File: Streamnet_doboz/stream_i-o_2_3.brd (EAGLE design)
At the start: 192 x 74.5 mm, 225 parts, among them IC1 SCT21SOP16, IC12 LD117AS33TR, IC3 BEM_VEDO, IC4 7805TV, J1 PIN1-2, Q1 20MHz, T1 BD242, T10 BD242, T11 BD242, T12 BD242, T13 BD242, T14 BD242, T15 BD242, T16 BD242, T17 BC858, T2 BD242, T3 BD242, T4 BD242, T5 BD242, T6 BD242, T7 BD242, T8 BD242, T9 BD242, U1 MAX232SOIC16, U2 PIC32MX250F128B-I_SS

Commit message: stream_haladás
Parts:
- removed U$2, U$3, U$4: SCT21SOP16, StarChips:SOP16
- added U$1, U$10, U$7, U$8, U$9: SCT2167SSOP, SCT2167:SSOP
- moved R16 288.9 mm to (-168.9, 33.8), flipped to the bottom
- moved D20 288.6 mm to (-168.8, 37.5), flipped to the bottom
- moved LED16 287.7 mm to (-168.3, 35.7), flipped to the bottom
- moved ZOLD_2P8 281.2 mm to (-165.0, 10.7), flipped to the bottom
- moved ZOLD_4P16 281.2 mm to (-165.0, 24.5), flipped to the bottom
- moved T16 273.7 mm to (-161.3, 27.3), flipped to the top
- moved D19 262.9 mm to (-155.9, 36.8), flipped to the bottom
- moved R46 259.1 mm to (-154.0, 2.22), flipped to the top
- moved R47 259.1 mm to (-154.0, 4.76), flipped to the top
- moved ZOLD_2P7 257.2 mm to (-153.0, 10.7), flipped to the bottom
- moved ZOLD_4P15 257.2 mm to (-153.0, 24.5), flipped to the bottom
- moved LED15 256.5 mm to (-152.7, 34.0), flipped to the bottom
- moved T15 253.4 mm to (-151.1, 38.7), flipped to the top
- moved D31 250.8 mm to (-149.9, 17.1), flipped to the top
- moved D32 250.8 mm to (-149.9, 14.8), flipped to the top
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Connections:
- removed net N$102: OK4.13, U$3.6
- removed net N$136: U$3.14, U$4.2
- new net 01_GND: U$10.1, U$7.1, U$8.1, U$9.1
- new net 16_VDD: U$10.16, U$7.16, U$8.16, U$9.16
- new net N$97: OK4.13, U$7.6
- net +3V3: now also U$1.16; no longer U$2.16, U$3.16, U$4.16
- net CHECK: no longer U$4.14
- net CLK: now also U$1.3; no longer U$2.3, U$3.3, U$4.3
- net GND: now also U$1.1, U$1.13; no longer U$2.1, U$2.13, U$3.1, U$3.13, U$4.1, U$4.13
- net LABE: now also U$1.4; no longer U$2.4, U$3.4, U$4.4
- net N$100: now also U$8.11; no longer U$4.11
- net N$101: now also U$7.5; no longer U$3.5
- net N$103: now also U$7.7; no longer U$3.7
- net N$104: now also U$7.8; no longer U$3.8
- net N$113: now also U$8.12; no longer U$4.12
- net N$127: now also U$8.5; no longer U$4.5
- net N$128: now also U$8.6; no longer U$4.6
- net N$129: now also U$8.7; no longer U$4.7
- net N$130: now also U$8.8; no longer U$4.8
- net N$131: no longer U$4.15
- net N$132: no longer U$3.15
- net N$133: now also U$1.15; no longer U$2.15
- net N$134: now also U$1.2; no longer U$2.2
- net N$135: now also U$1.14; no longer U$2.14, U$3.2
- net N$64: now also U$1.9; no longer U$2.9
- net N$65: now also U$1.10; no longer U$2.10
- net N$66: now also U$1.11; no longer U$2.11
- net N$67: now also U$1.12; no longer U$2.12
- net N$76: now also U$8.9; no longer U$4.9
- net N$77: now also U$1.5; no longer U$2.5
- net N$78: now also U$1.6; no longer U$2.6
- net N$79: now also U$1.7; no longer U$2.7
- net N$80: now also U$1.8; no longer U$2.8
- net N$88: now also U$7.9; no longer U$3.9
- net N$89: now also U$7.10; no longer U$3.10
- net N$90: now also U$7.11; no longer U$3.11
- net N$91: now also U$7.12; no longer U$3.12
- net N$96: now also U$8.10; no longer U$4.10
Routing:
- net LABE: track 302.0 -> 142.3 mm, vias 5 -> 2
- net N$135: track 124.6 -> 0.00 mm, vias 2 -> 0
- net N$136: track 115.8 -> 0.00 mm, vias 2 -> 0
- net GND: track 909.1 -> 899.7 mm
- net +3V3: track 376.9 -> 367.8 mm
- net N$102: track 5.63 -> 0.00 mm
- net N$97: track 0.00 -> 5.04 mm
- net CLK: track 280.3 -> 276.1 mm
- net N$130: track 7.50 -> 3.89 mm
- net N$103: track 6.90 -> 3.61 mm
- net N$79: track 6.90 -> 3.77 mm
- net N$133: track 11.6 -> 9.51 mm
- net N$132: track 3.95 -> 2.08 mm
- net N$131: track 4.80 -> 3.30 mm
- net N$89: track 40.4 -> 39.0 mm
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- added copper zone on layer 1, net GND
- removed copper zone on layer 16, net GND
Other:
- board size 192 x 74.5 mm -> 287 x 74.5 mm

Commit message: streamnet ssopsodott
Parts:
- removed IC1, U$5: SCT21SOP16, StarChips:SOP16
- added D43, D44, D45, D46, D47, D48, D49, D50, D51, D52, D53, D54, D55, D56, D57, D58: (no value), dp_devices:SOD-123
- moved R16 272.4 mm to (103.5, 36.7), flipped to the top
- moved D20 272.1 mm to (103.3, 40.3), flipped to the top
- moved LED16 271.2 mm to (102.9, 38.6), flipped to the top
- moved U$8 267.2 mm to (70.3, 14.1), flipped to the bottom
- moved ZOLD_2P8 264.7 mm to (99.6, 13.6), flipped to the top
- moved ZOLD_4P16 264.7 mm to (99.6, 27.4), flipped to the top
- moved U$10 261.9 mm to (46.4, 32.4), flipped to the bottom, turned to 180 degrees
- moved U$7 260.0 mm to (70.5, 29.4), flipped to the bottom
- moved T16 257.2 mm to (95.9, 30.2), flipped to the bottom
- moved D19 246.4 mm to (90.5, 39.7), flipped to the top
- moved R46 242.6 mm to (88.6, 5.08), flipped to the bottom
- moved R47 242.6 mm to (88.6, 7.62), flipped to the bottom
- moved ZOLD_2P7 240.7 mm to (87.6, 13.6), flipped to the top
- moved ZOLD_4P15 240.7 mm to (87.6, 27.4), flipped to the top
- moved LED15 240.0 mm to (87.3, 36.8), flipped to the top
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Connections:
- removed net 01_GND: U$10.1, U$7.1, U$8.1, U$9.1
- removed net 16_VDD: U$10.16, U$7.16, U$8.16, U$9.16
- removed net GND: C10.2, C11.2, C12.2, C13.2, C14.2, C15.2, C16.2, C17.2, C4.2, C5.2, C6.1, C7.1, C8.-, C9.2, D41.A, D42.A, DC1.1, IC1.1, IC1.13, IC12.1, IC4.2, R17.1, R18.1, R43.1, R48.1, R49.1, R50.1, R51.1, R56.1, R67.2, SV1.1, U$1.1, U$1.13, U$5.1, U$5.13, U$6.6A, U$6.7A, U1.15, U2.19, U2.27, U2.8, ZOLD_2P1.1, ZOLD_2P2.1, ZOLD_2P3.1, ZOLD_2P4.1, ZOLD_2P5.1, ZOLD_2P6.1, ZOLD_2P7.1, ZOLD_2P8.1, ZOLD_3P1.1, ZOLD_3P2.1, ZOLD_4P1.1, ZOLD_4P1.3, ZOLD_4P10.1, ZOLD_4P10.3, ZOLD_4P11.1, ZOLD_4P11.3, ZOLD_4P12.1, ZOLD_4P12.3, ZOLD_4P13.1, ZOLD_4P13.3, ZOLD_4P14.1, ZOLD_4P14.3, ZOLD_4P15.1, ZOLD_4P15.3, ZOLD_4P16.1, ZOLD_4P16.3, ZOLD_4P17.1, ZOLD_4P2.1, ZOLD_4P2.3, ZOLD_4P3.1, ZOLD_4P3.3, ZOLD_4P4.1, ZOLD_4P4.3, ZOLD_4P5.1, ZOLD_4P5.3, ZOLD_4P6.1, ZOLD_4P6.3, ZOLD_4P7.1, ZOLD_4P7.3, ZOLD_4P8.1, ZOLD_4P8.3, ZOLD_4P9.1, ZOLD_4P9.3
- removed net N$131: R51.2
- removed net N$133: R49.2, U$1.15
- new net N$102: R50.1, U$7.15
- new net N$136: U$7.14, U$8.2
- new net N$156: R17.1, U$9.15
- new net N$171: R18.2, U$10.15
- net +3V3: now also U$10.16, U$7.16, U$8.16, U$9.16; no longer IC1.16, U$5.16
- net CHECK: now also U$8.13
- net CLK: now also U$10.3, U$7.3, U$8.3, U$9.3; no longer IC1.3, U$5.3
- net LABE: now also U$7.4, U$8.4
- net LAKI: now also U$10.4, U$9.4; no longer IC1.4, U$5.4
- net N$1: now also U$9.8; no longer IC1.8
- net N$10: now also D45.C
- net N$12: now also D46.C
- net N$13: now also U$9.9; no longer IC1.9
- net N$132: now also R51.1, U$8.15; no longer R50.2
- net N$134: now also U$10.14; no longer U$5.14
- net N$135: now also U$7.2
- net N$15: now also D47.C
- net N$16: now also U$9.10; no longer IC1.10
- net N$18: now also D48.C
- net N$19: now also U$9.11; no longer IC1.11
- net N$2: now also U$9.5; no longer IC1.5
- net N$21: now also D49.C
- net N$22: now also U$9.12; no longer IC1.12
- net N$24: now also D50.C
- net N$25: now also R49.1, U$1.15; no longer IC1.15, R17.2
- net N$26: now also C10.2, C11.2, C12.2, C13.2, C14.2, C15.2, C16.2, C17.2, C4.2, C5.2, C6.1, C7.1, C8.-, C9.2, D41.A, D42.A, D43.A, D44.A, D45.A, D46.A, D47.A, D48.A, D49.A, D50.A, D51.A, D52.A, D53.A, D54.A, D55.A, D56.A, D57.A, D58.A, DC1.1, IC12.1, IC4.2, R17.2, R18.1, R43.1, R48.1, R49.2, R50.2, R51.2, R56.1, R67.2, SV1.1, U$1.1, U$1.13, U$10.1, U$10.13, U$6.6A, U$6.7A, U$7.1, U$7.13, U$8.1, U$8.14, U$9.1, U$9.13, U1.15, U2.19, U2.27, U2.8, ZOLD_2P1.1, ZOLD_2P2.1, ZOLD_2P3.1, ZOLD_2P4.1, ZOLD_2P5.1, ZOLD_2P6.1, ZOLD_2P7.1, ZOLD_2P8.1, ZOLD_3P1.1, ZOLD_3P2.1, ZOLD_4P1.1, ZOLD_4P1.3, ZOLD_4P10.1, ZOLD_4P10.3, ZOLD_4P11.1, ZOLD_4P11.3, ZOLD_4P12.1, ZOLD_4P12.3, ZOLD_4P13.1, ZOLD_4P13.3, ZOLD_4P14.1, ZOLD_4P14.3, ZOLD_4P15.1, ZOLD_4P15.3, ZOLD_4P16.1, ZOLD_4P16.3, ZOLD_4P17.1, ZOLD_4P2.1, ZOLD_4P2.3, ZOLD_4P3.1, ZOLD_4P3.3, ZOLD_4P4.1, ZOLD_4P4.3, ZOLD_4P5.1, ZOLD_4P5.3, ZOLD_4P6.1, ZOLD_4P6.3, ZOLD_4P7.1, ZOLD_4P7.3, ZOLD_4P8.1, ZOLD_4P8.3, ZOLD_4P9.1, ZOLD_4P9.3; no longer R18.2, U$5.15
- net N$27: now also U$10.2, U$9.14; no longer IC1.14, U$5.2
- net N$33: now also U$10.5; no longer U$5.5
- net N$35: now also D51.C
- net N$36: now also U$10.6; no longer U$5.6
- net N$38: now also D52.C
- net N$39: now also U$10.7; no longer U$5.7
- net N$4: now also D43.C
- net N$41: now also D53.C
- net N$42: now also U$10.8; no longer U$5.8
- net N$44: now also D54.C
- net N$45: now also U$10.9; no longer U$5.9
- net N$47: now also D55.C
- net N$48: now also U$10.10; no longer U$5.10
- net N$5: now also U$9.6; no longer IC1.6
- net N$50: now also D56.C
- net N$51: now also U$10.11; no longer U$5.11
- net N$53: now also D57.C
- net N$54: now also U$10.12; no longer U$5.12
- net N$56: now also D58.C
- net N$7: now also D44.C
- net N$8: now also U$9.7; no longer IC1.7
- net SDO1: now also U$9.2; no longer IC1.2
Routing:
- net GND: track 899.7 -> 0.00 mm, vias 16 -> 0
- net N$26: track 4.77 -> 880.7 mm, vias 0 -> 18
- net LABE: track 142.3 -> 270.4 mm, vias 2 -> 5
- net N$135: track 0.00 -> 115.6 mm, vias 0 -> 2
- net N$136: track 0.00 -> 22.0 mm, vias 0 -> 2
- net +3V3: track 367.8 -> 387.7 mm, vias 9 -> 11
- net CLK: track 276.1 -> 288.9 mm
- net N$133: track 9.51 -> 0.00 mm
- net N$171: track 0.00 -> 7.49 mm
- net N$102: track 0.00 -> 7.07 mm, vias 0 -> 1
- net N$130: track 3.89 -> 9.35 mm
- net N$79: track 3.77 -> 8.43 mm
- net N$103: track 3.61 -> 7.72 mm
- net N$27: track 104.3 -> 108.0 mm
- net SDO1: track 39.6 -> 43.2 mm
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- added copper zone on layer 16, net N$26
- removed copper zone on layer 1, net GND
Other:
- board size 287 x 74.5 mm -> 202.4 x 71.6 mm

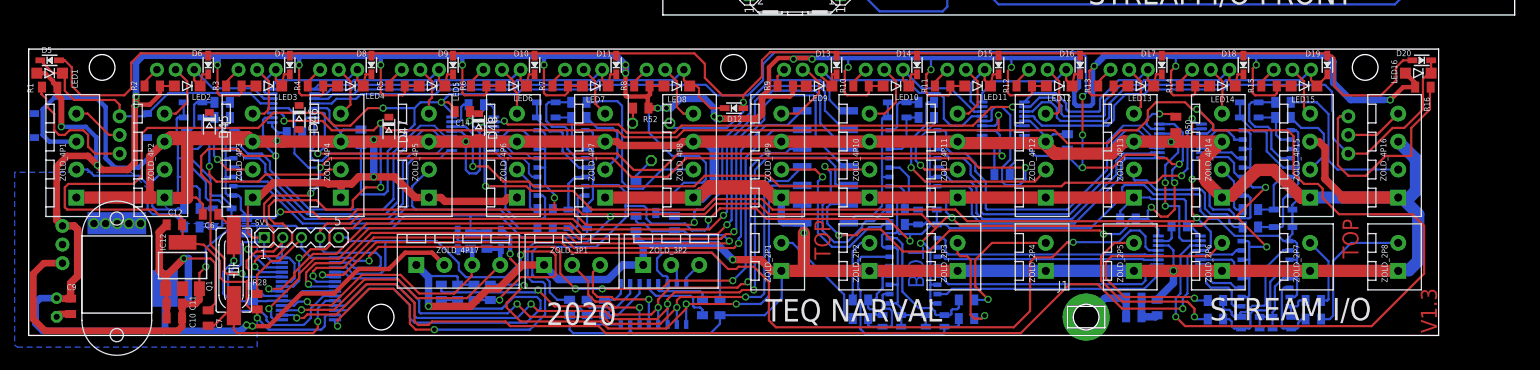
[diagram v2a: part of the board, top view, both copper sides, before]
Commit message: stream testatkot megszunt
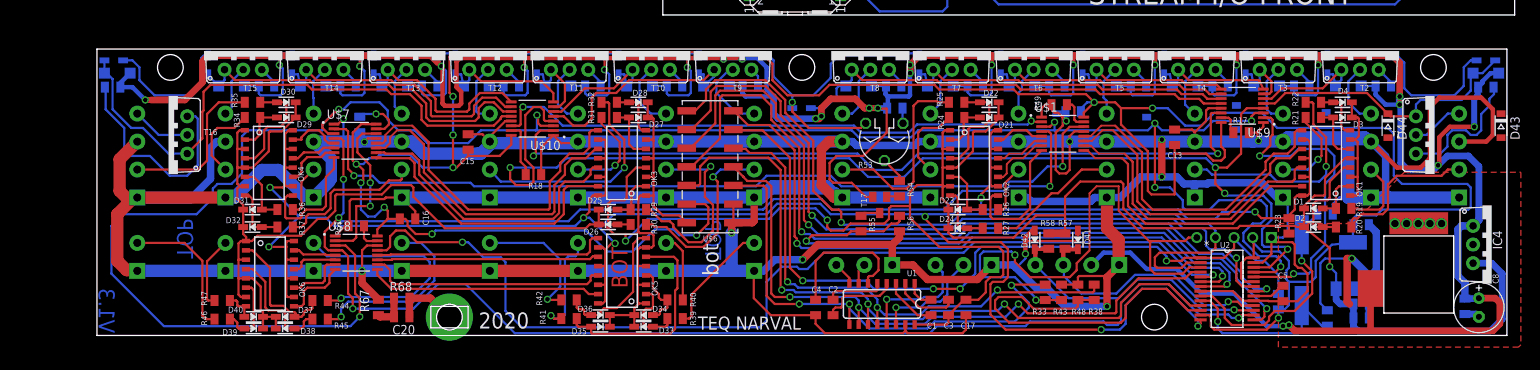
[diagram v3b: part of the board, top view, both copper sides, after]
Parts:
- moved D43 199.7 mm to (114.1, 31.4), flipped to the top
- moved IC4 197.2 mm to (112.9, 15.2), flipped to the top
- moved D5 195.6 mm to (112.1, 40.3), flipped to the bottom
- moved LED1 195.6 mm to (112.1, 38.6), flipped to the bottom
- moved R1 195.6 mm to (112.1, 36.7), flipped to the bottom
- moved C8 193.7 mm to (111.1, 6.67), flipped to the top
- moved C9 189.9 mm to (109.2, 6.83), flipped to the bottom
- moved ZOLD_4P1 189.3 mm to (108.9, 27.4), flipped to the bottom
- moved T1 181.6 mm to (105.1, 30.2), flipped to the top
- moved R16 178.4 mm to (-74.9, 36.7), flipped to the bottom
- moved D20 178.1 mm to (-74.8, 40.3), flipped to the bottom
- moved DC1 177.3 mm to (102.9, 11.2), flipped to the bottom
- moved LED16 177.2 mm to (-74.3, 38.6), flipped to the bottom
- moved ZOLD_2P8 170.7 mm to (-71.1, 13.6), flipped to the bottom
- moved ZOLD_4P16 170.7 mm to (-71.1, 27.4), flipped to the bottom
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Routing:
- net U2RX: track 61.6 -> 74.3 mm
- net N$26: track 880.7 -> 890.6 mm
- net +5V: track 431.0 -> 438.3 mm
- net N$75: track 24.2 -> 18.1 mm
- added copper zone on layer 1, net N$26
- removed copper zone on layer 16, net N$26
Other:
- board size 202.4 x 71.6 mm -> 193.1 x 71.6 mm
- board text removed: "GND ATKOT"
